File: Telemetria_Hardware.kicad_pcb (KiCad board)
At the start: 2 copper layers, 81.3 x 87.6 mm, 16 parts, among them M100A 1715734

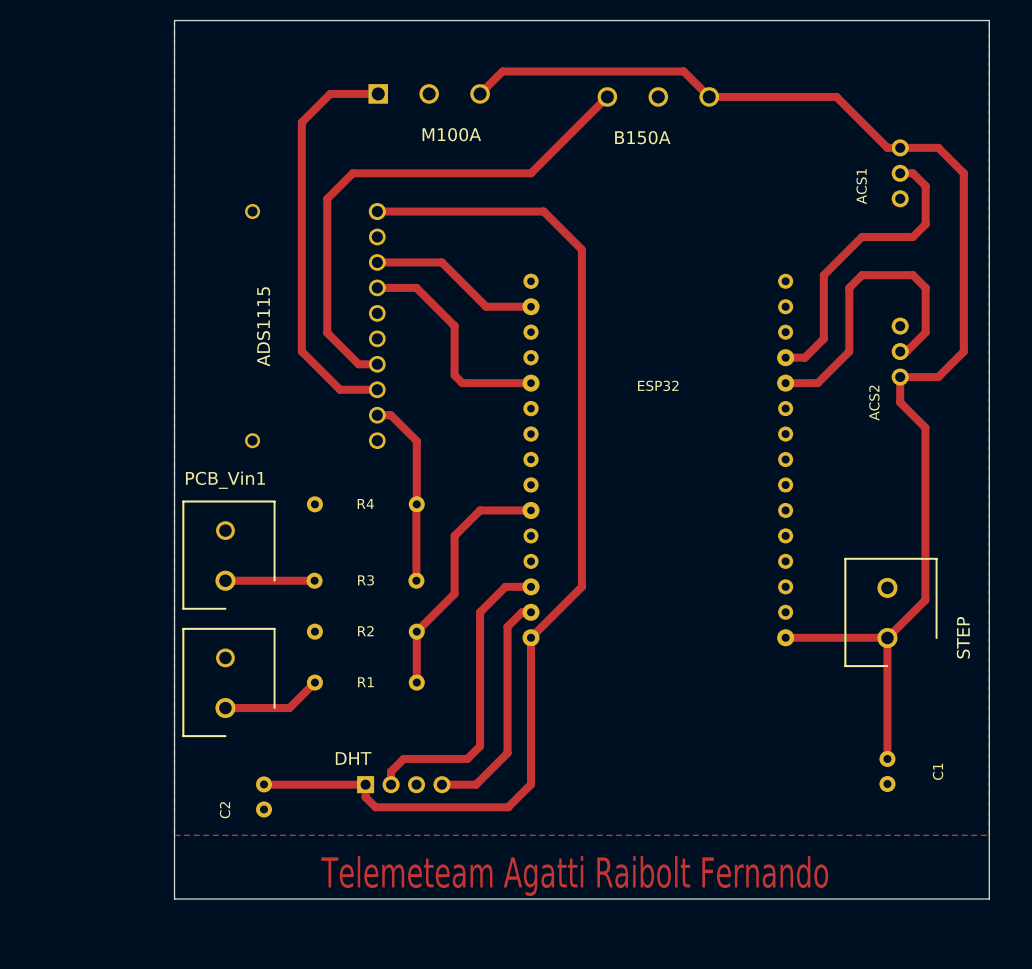
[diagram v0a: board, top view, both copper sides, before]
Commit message: Mudanças pré DSB 2024
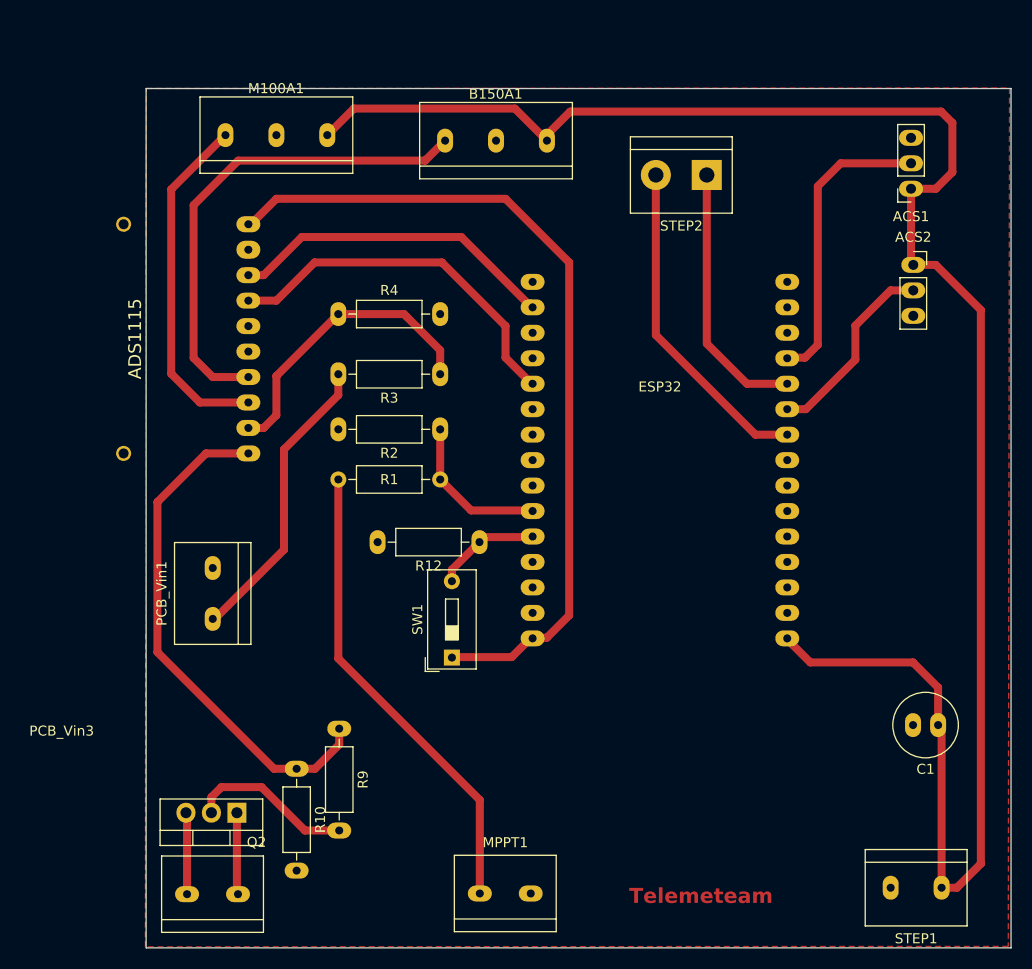
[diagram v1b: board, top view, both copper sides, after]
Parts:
- removed B150A, M100A: 1715734, Terminal_Block_PCB_3Way:Connector_KRE_3W_5,08mm
- removed C2: C_Polarized, Capacitor_THT:C_Radial_D6.3mm_H11.0mm_P2.50mm
- removed DHT: Conn_01x04_Female, Connector_PinSocket_2.54mm:PinSocket_1x04_P2.54mm_Vertical
- removed MPPT, STEP: CTB1202_2BK, Terminal_Block_PCB_2Way:KRE_Terminal_2Way_5.08mm
- added B150A1: 1715734, TerminalBlock:TerminalBlock_bornier-3_P5.08mm, F.Cu at (95.6, 57.7)
- added M100A1: 1715734, TerminalBlock:TerminalBlock_bornier-3_P5.08mm, F.Cu at (73.7, 57.1)
- added MPPT1: CTB1202_2BK, TerminalBlock:TerminalBlock_bornier-2_P5.08mm, F.Cu at (99.0, 132.8)
- added PCB_Vin3: CTB1202_2BK, TerminalBlock:TerminalBlock_bornier-2_P5.08mm, F.Cu at (69.8, 132.9)
- added Q2: TIP120, Package_TO_SOT_THT:TO-220-3_Vertical, F.Cu at (74.8, 124.7)
- added R10: 130Ω, Resistor_THT:R_Axial_DIN0207_L6.3mm_D2.5mm_P10.16mm_Horizontal, F.Cu at (80.8, 120.4)
- added R12: R, Resistor_THT:R_Axial_DIN0207_L6.3mm_D2.5mm_P10.16mm_Horizontal, F.Cu at (99.0, 97.8)
- added R9: 39Ω, Resistor_THT:R_Axial_DIN0207_L6.3mm_D2.5mm_P10.16mm_Horizontal, F.Cu at (85.0, 116.4)
- added STEP1: CTB1202_2BK, TerminalBlock:TerminalBlock_bornier-2_P5.08mm, F.Cu at (145.1, 132.2)
- added STEP2: CTB1202_2BK, TerminalBlock:TerminalBlock_bornier-2_P5.08mm, F.Cu at (121.7, 61.1)
- added SW1: SW_SPST, Button_Switch_THT:SW_DIP_SPSTx01_Slide_9.78x4.72mm_W7.62mm_P2.54mm, F.Cu at (96.2, 109.3)
- ACS1, ACS2, C1, R1, R2, R3, R4: moved to F.Cu
- ESP32: footprint esp32_devkit_v1_doit:esp32_devkit_v1_doit -> ESP32:esp32_devkit_v1_doit
- PCB_Vin1: footprint Terminal_Block_PCB_2Way:KRE_Terminal_2Way_5.08mm -> TerminalBlock:TerminalBlock_bornier-2_P5.08mm
- moved R2 23.7 mm to (95.1, 86.5), turned to 180 degrees
- moved R3 20.7 mm to (95.1, 81.0)
- moved R4 20.5 mm to (84.9, 75.0), turned to 0 degrees
- moved R1 20.4 mm to (95.1, 91.5)
- moved ADS1115 12.9 mm to (75.9, 66.0)
- moved ACS2 11.3 mm to (142.3, 70.1)
- moved C1 6.08 mm to (144.8, 116.0), turned to 180 degrees
- moved ACS1 4.22 mm to (142.1, 62.5)
- moved PCB_Vin1 4.02 mm to (72.4, 105.4)
- moved ESP32 0.17 mm to (117.0, 71.8)
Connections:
- ACS2 pad 2: Net-(ACS2-Pad2) -> Net-(ACS2-Pin_2)
- ADS1115 pad 10: unconnected-(ADS1115-Pad10) -> Net-(ADS1115-A3)
- ESP32 pad 12: unconnected-(ESP32-Pad12) -> Net-(ESP32-IO12)
- ESP32 pad 13: unconnected-(ESP32-Pad13) -> Net-(ESP32-IO13)
- ESP32 pad 18: Net-(DHT1-Pad2) -> unconnected-(ESP32-IO15-Pad18)
- ESP32 pad 20: unconnected-(ESP32-Pad20) -> Net-(ESP32-IO4)
- ESP32 pad 21: Net-(ESP32-Pad21) -> Net-(ESP32-IO16)
- ESP32 pad 5: Net-(ACS2-Pad2) -> Net-(ESP1-IO35)
- ESP32 pad 6: unconnected-(ESP32-Pad6) -> Net-(ACS2-Pin_2)
- ESP32 pad 7: unconnected-(ESP32-Pad7) -> Net-(ESP1-IO33)
- ESP32 pad 8: unconnected-(ESP32-Pad8) -> Net-(ESP32-IO25)
- R1 pad 1: Net-(ESP32-Pad21) -> Net-(ESP1-IO16)
- R2 pad 1: GND -> Net-(ESP1-IO16)
- R2 pad 2: Net-(ESP32-Pad21) -> GND
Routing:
- net Net-(ACS1-Pin_1): track 129.5 -> 190.9 mm
- net Net-(ADS1115-A3): track 0.00 -> 51.6 mm
- net Net-(MPPT1-Pad1): track 9.98 -> 47.1 mm
- net Net-(ESP1-IO33): track 0.00 -> 33.2 mm
- net Net-(DHT1-Pad2): track 30.7 -> 0.00 mm
- net Net-(ACS2-Pad2): track 30.5 -> 0.00 mm
- net Net-(ESP1-IO35): track 0.00 -> 26.5 mm
- net Net-(ESP32-Pad21): track 24.9 -> 0.00 mm
- net GND: track 23.4 -> 0.00 mm
- net Net-(ADS1115-VDD): track 106.7 -> 84.3 mm
- net Net-(PCB_Vin1-Pad1): track 8.93 -> 29.7 mm
- net Net-(ACS2-Pin_2): track 0.00 -> 19.5 mm
- net Net-(ADS1115-SCL): track 17.2 -> 33.0 mm
- net Net-(Q2-C): track 0.00 -> 15.4 mm
- net Net-(ESP32-IO16): track 0.00 -> 15.3 mm
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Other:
- board size 81.3 x 87.6 mm -> 86.3 x 85.7 mm
- board text added: "Telemeteam"
- board text removed: "Telemeteam Agatti Raibolt Fernando"
